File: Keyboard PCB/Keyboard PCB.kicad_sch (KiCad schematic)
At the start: 9 parts, among them SW1 SW_Push, SW2 SW_Push, SW3 SW_Push, SW4 SW_Push, SW5 SW_Push, SW6 SW_Push, U1 MOUDLE-SEEEDUINO-XIAO

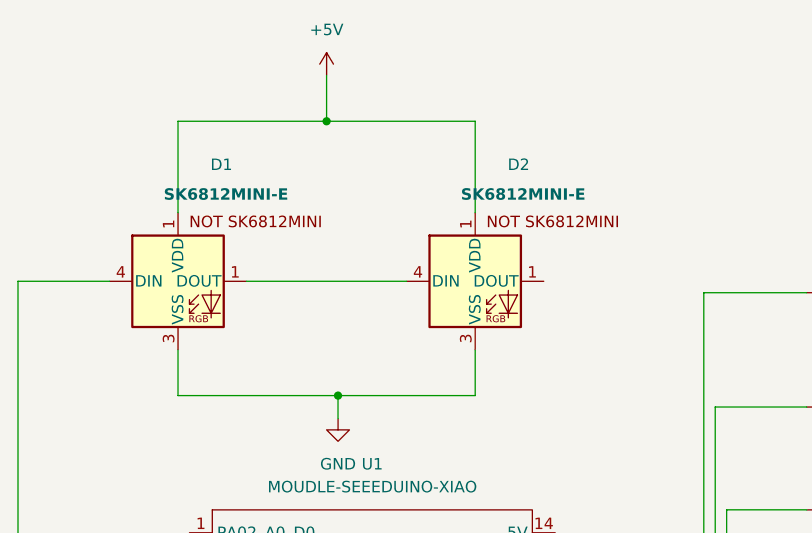
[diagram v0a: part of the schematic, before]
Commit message: Who needs autosaves?
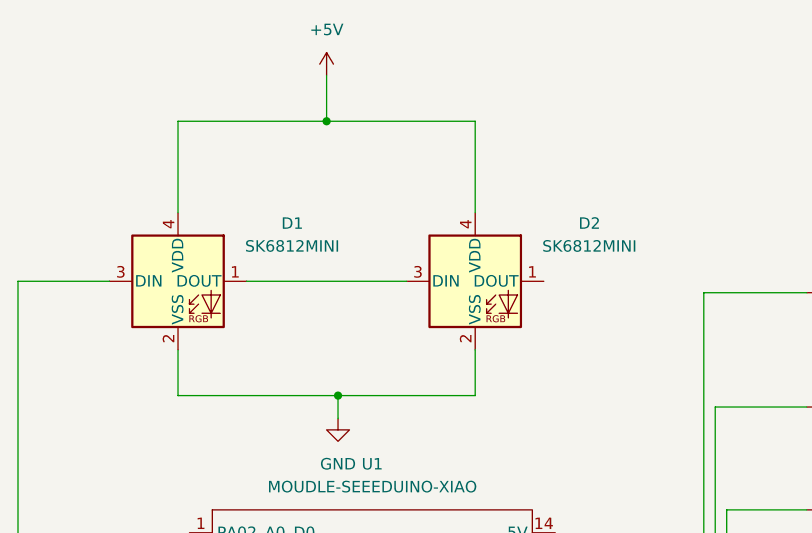
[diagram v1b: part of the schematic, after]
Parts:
- removed D1, D2: SK6812MINI-E, footprints:SK6812MINI-E_fixed, symbol SK6812MINI-E:SK6812MINI-E
- added D1, D2: SK6812MINI, LED_SMD:LED_SK6812MINI_PLCC4_3.5x3.5mm_P1.75mm, symbol LED:SK6812MINI
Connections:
- net +5V: now also D1.4 (VDD), D2.4 (VDD)
- net GND: now also D1.2 (VSS), D2.2 (VSS)
- net at U1.5 (PA8_A4_D4_SDA): now also D1.3 (DIN)
- new net: D1.1 (DOUT), D2.3 (DIN)
